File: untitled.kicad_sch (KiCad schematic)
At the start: 34 parts, among them Q2 NMOS, Q3 NMOS, U4 TLV3501AID, U5 DGS0010A, U6 OPA2392, U7 ADC10065

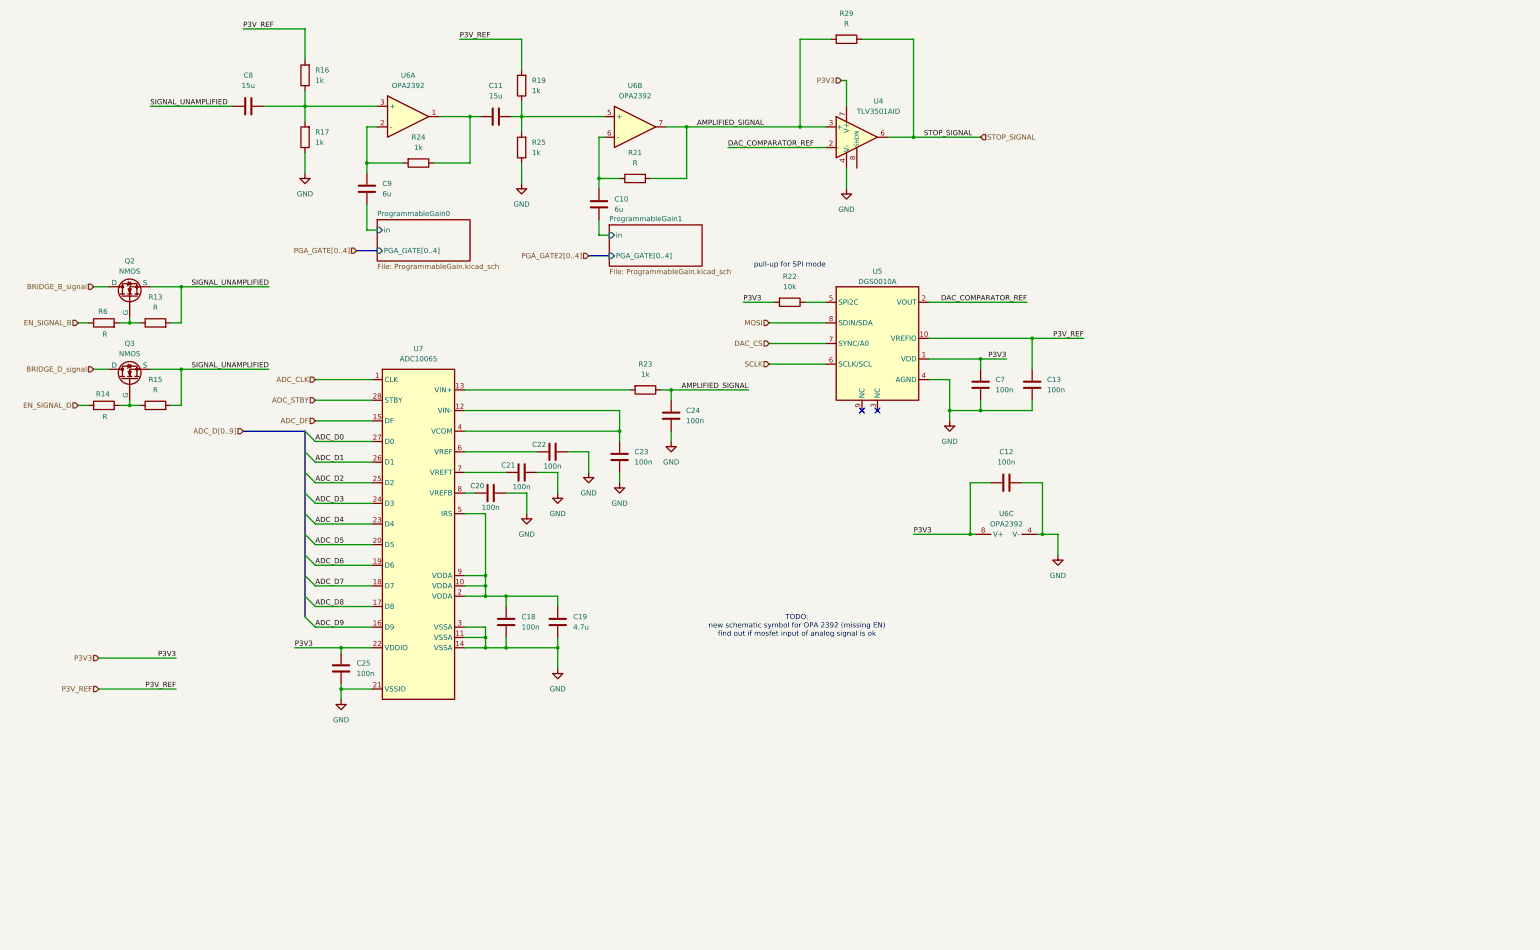
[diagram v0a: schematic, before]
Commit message: schematics done
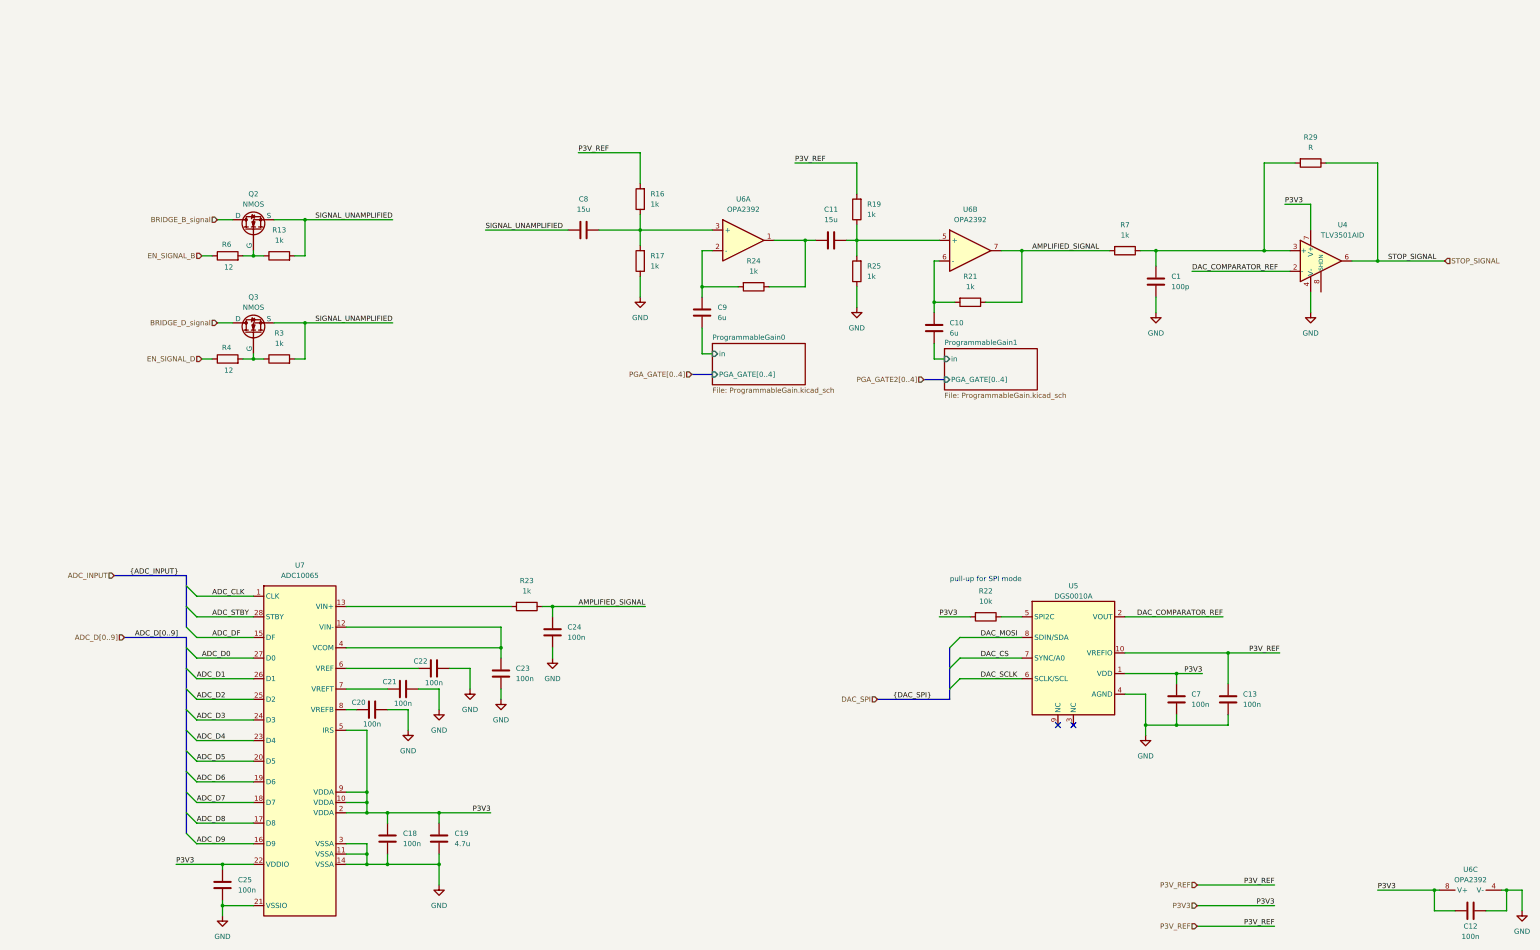
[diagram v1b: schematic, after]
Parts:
- removed R14, R15: R, symbol Device:R
- added C1: 100p, Capacitor_SMD:C_0603_1608Metric_Pad1.08x0.95mm_HandSolder, symbol Device:C
- added R3, R7: 1k, Resistor_SMD:R_0603_1608Metric_Pad0.98x0.95mm_HandSolder, symbol Device:R
- added R4: 12, Resistor_SMD:R_0603_1608Metric_Pad0.98x0.95mm_HandSolder, symbol Device:R
- R13, R21: value R -> 1k; footprint (none) -> Resistor_SMD:R_0603_1608Metric_Pad0.98x0.95mm_HandSolder
- R6: value R -> 12; footprint (none) -> Resistor_SMD:R_0603_1608Metric_Pad0.98x0.95mm_HandSolder
- U6: footprint (none) -> Package_SO:SOIC-8_3.9x4.9mm_P1.27mm
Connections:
- net AMPLIFIED_SIGNAL: now also R7.2; no longer R29.2, U4.3 (+)
- net EN_SIGNAL_D: now also R4.1
- net GND: now also C1.1
- net P3V3: now also C18.2, C19.2, U7.10 (VDDA), U7.2 (VDDA), U7.5 (IRS), U7.9 (VDDA)
- net SIGNAL_UNAMPLIFIED: now also R3.2
- net at Q3.2 (G): now also R3.1, R4.2
- net MOSI renamed DAC_MOSI
- net SCLK renamed DAC_SCLK
- new net: C1.2, R29.2, R7.1, U4.3 (+)
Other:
- note removed: "TODO: new schematic symbol for OPA 2392 (missing EN) find out if mosfet input of analog signal is ok"
- moved on the sheet: C10, C11, C12, C13, C18, C19, C20, C21, C22, C23, C24, C25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
